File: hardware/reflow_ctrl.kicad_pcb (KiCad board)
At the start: 2 copper layers, 160 x 100 mm, 36 parts, among them IC1 MAX6675, IC2 ATXMEGA128A4U-A, P1 PDI, U1 LT1129CST-3.3, U2 MOC3063, U3 BTA41/600B, X1 USB-Mini-B, X2 Mains, X3 Load, X4 Thermocouple

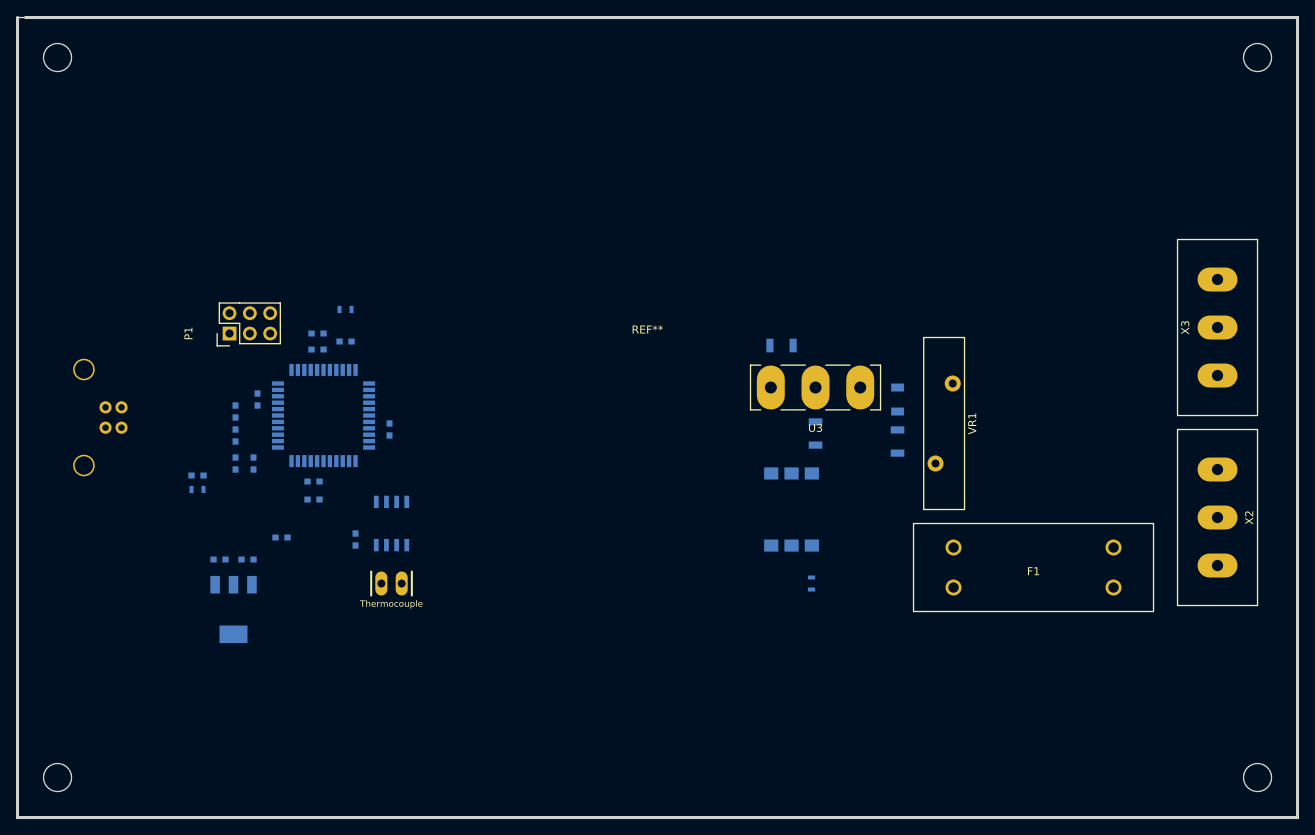
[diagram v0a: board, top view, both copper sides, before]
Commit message: Update board
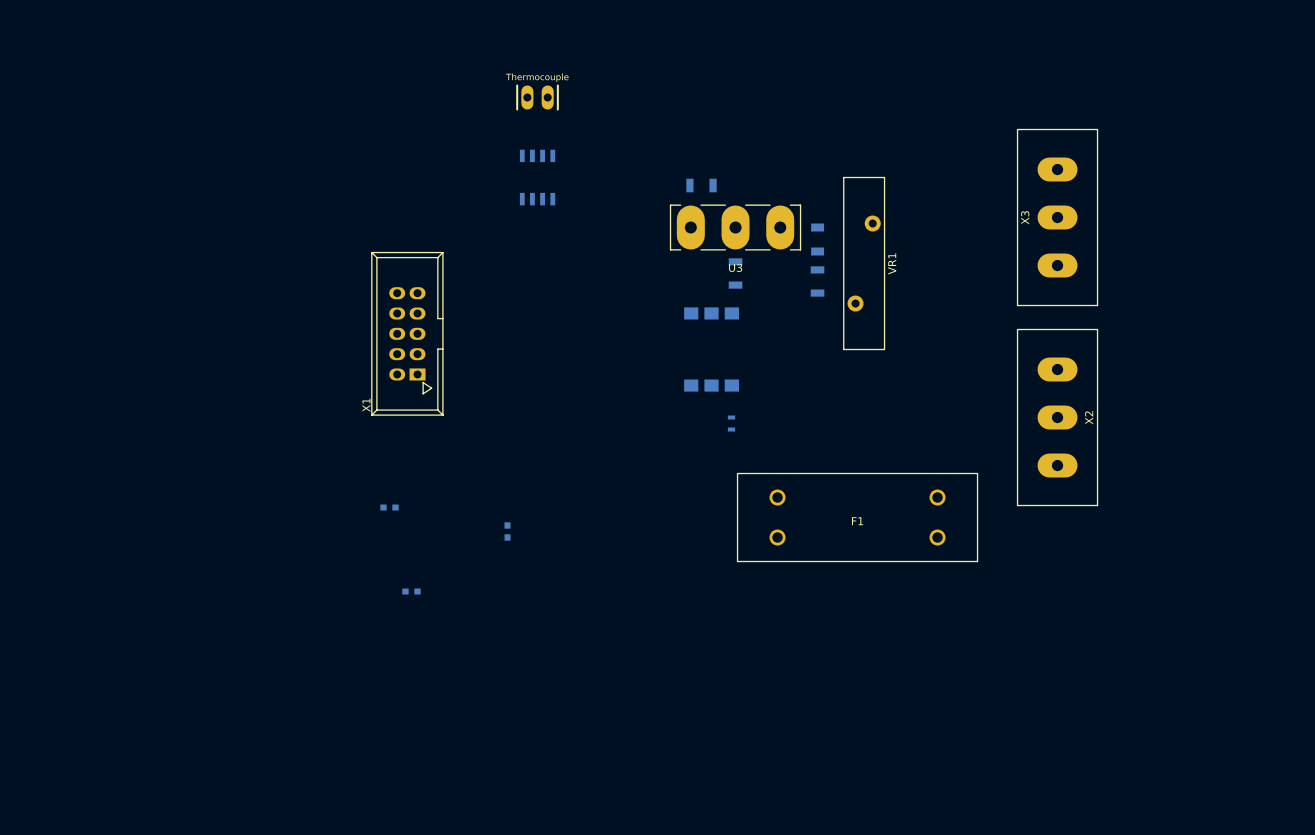
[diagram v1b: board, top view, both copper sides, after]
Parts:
- removed C10, C4, C5, L1: 10u, Capacitors_SMD:C_0603
- removed C3, C6, C7, C8, C9: 100n, Capacitors_SMD:C_0603
- removed D1, D2, D3: TVS 5V, Capacitors_SMD:C_0603
- removed IC2: ATXMEGA128A4U-A, Housings_QFP:TQFP-44_10x10mm_Pitch0.8mm
- removed L2: Bead 1k@100MHz, Capacitors_SMD:C_0603
- removed P1: PDI, Pin_Headers:Pin_Header_Straight_2x03
- removed R1: 1M, Resistors_SMD:R_0603
- removed R2: 10k, Resistors_SMD:R_0603
- removed REF**: EuroBoard160mmX100mm_holes, EuroBoard_Outline:EuroBoard160mmX100mm_holes
- removed U1: LT1129CST-3.3, uMIDI:SOT-223
- C1: value 4.7n -> 100n
- C2: value 10u -> 100n
- X1: value USB-Mini-B -> Master; footprint Connect:USB_B -> uMIDI:Con-boxed_header-THT; moved to F.Cu
- moved X4 63.4 mm to (125.0, 60.0), turned to 180 degrees
- moved IC1 46.9 mm to (125.0, 70.0), turned to 270 degrees
- moved X1 36.9 mm to (108.7, 89.5), turned to 90 degrees
- moved C1 24.3 mm to (106.5, 111.2)
- moved C2 24.3 mm to (109.2, 121.8)
- moved X3 24.3 mm to (190.0, 75.0)
- moved X2 23.6 mm to (190.0, 100.0)
- moved F1 22.9 mm to (165.0, 112.5)
- moved C12 22.4 mm to (160.0, 77.8)
- moved R3 22.4 mm to (149.2, 100.8)
- moved R4 22.4 mm to (149.8, 82.0)
- moved R5 22.4 mm to (145.5, 71.0)
- moved R6 22.4 mm to (160.0, 83.0)
- moved U2 22.4 mm to (146.8, 91.5)
- moved U3 22.4 mm to (149.8, 76.2)
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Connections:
- C1 pad 1: Net-(C1-Pad1) -> +3V3
- C11 pad 1: +5V -> +3V3
- C2 pad 1: VBUS -> +3V3
- IC1 pad 4: +5V -> +3V3
- X1 pad 1: VBUS -> +3V3
- X1 pad 2: /USB_p -> (no net)
- X1 pad 3: /USB_n -> (no net)
- X1 pad 4: GND -> (no net)
- X1 pad 5: Net-(C1-Pad1) -> /TC_SO
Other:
- board outline removed
